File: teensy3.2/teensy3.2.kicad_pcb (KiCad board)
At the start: 2 copper layers, 69 x 34 mm, 33 parts, among them J1 USB_B_Micro, J2 Conn_01x26, J3 Conn_01x26, SW1 Prog, U1 LP38691SD-3.3, U2 MKL02Z32VFG4, U3 MK20DX256VLH7, Y1 32.768 KHz, Y2 16 MHz

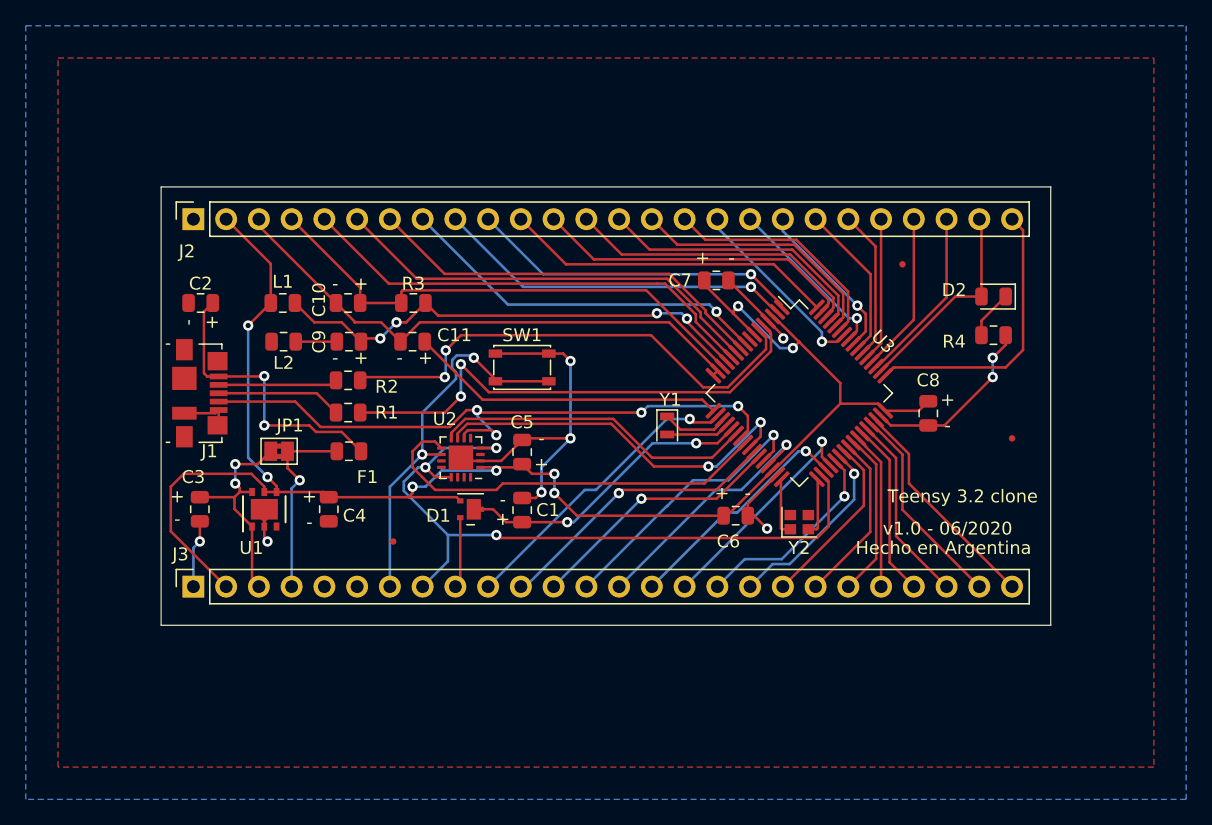
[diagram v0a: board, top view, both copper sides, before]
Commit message: ajustes para revision final
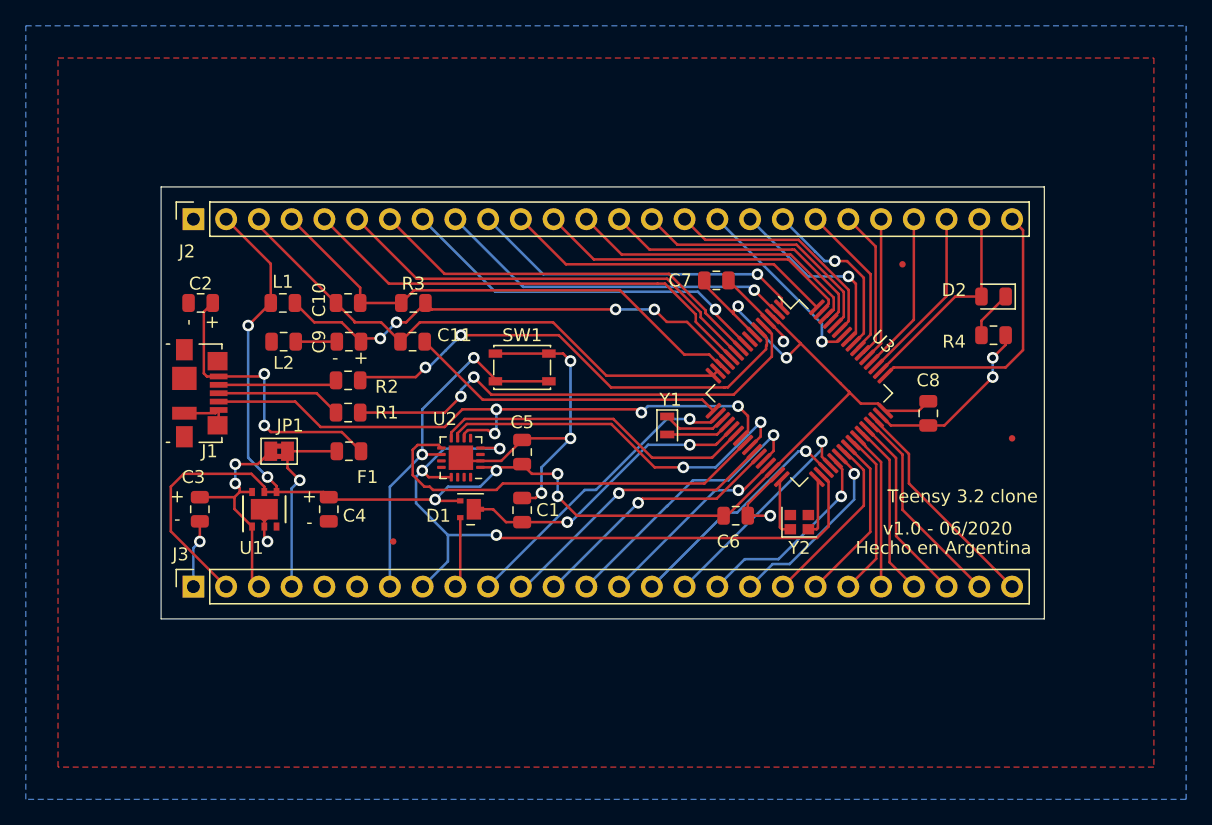
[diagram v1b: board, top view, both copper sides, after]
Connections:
- net /LED renamed Net-(D2-Pad2)
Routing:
- net /J2_14: track 19.7 -> 15.5 mm
- net Net-(J2-Pad18): track 13.4 -> 14.8 mm
- net /USB0_DM: track 38.7 -> 37.6 mm
- net /PROG: track 30.0 -> 29.0 mm
- net Net-(J2-Pad19): track 12.7 -> 13.6 mm
- net +3V3: track 129.3 -> 128.5 mm
- net /USB0_DP: track 39.3 -> 38.6 mm
- net /PTA1: track 50.6 -> 49.9 mm
- net /AREF: track 40.2 -> 39.7 mm
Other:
- board size 69 x 34 mm -> 68.5 x 33.5 mm
- net class Default: via_dia 0.8 -> 0.9; via_drill 0.4 -> 0.5
- rule trace_min: 0.1016 -> 0.2
- rule via_min_size: 0.4 -> 0.5
- board text added: "Mínimos (Mayer 8 mils): Grillas: 0. 5mm, 0.25 mm Vía: 0.8 mm (0.4 mm) Margen: 0.18 mm Pista: 0.20 mm Dist. a borde: 0.50 mm Terminación: HASL"
- board text removed: "Mínimos (Mayer 8 mils): Grillas: 0. 5mm, 0.25 mm Vía: 0.8 mm (0.4 mm) Margen: 0.18 mm Pista: 0.20 mm Dist. a borde: 0.30 mm Terminación: HASL"
